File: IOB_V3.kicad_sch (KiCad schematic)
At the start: 6 parts, among them J1 Conn_01x02, J2 Conn_01x03, U1 REF3033

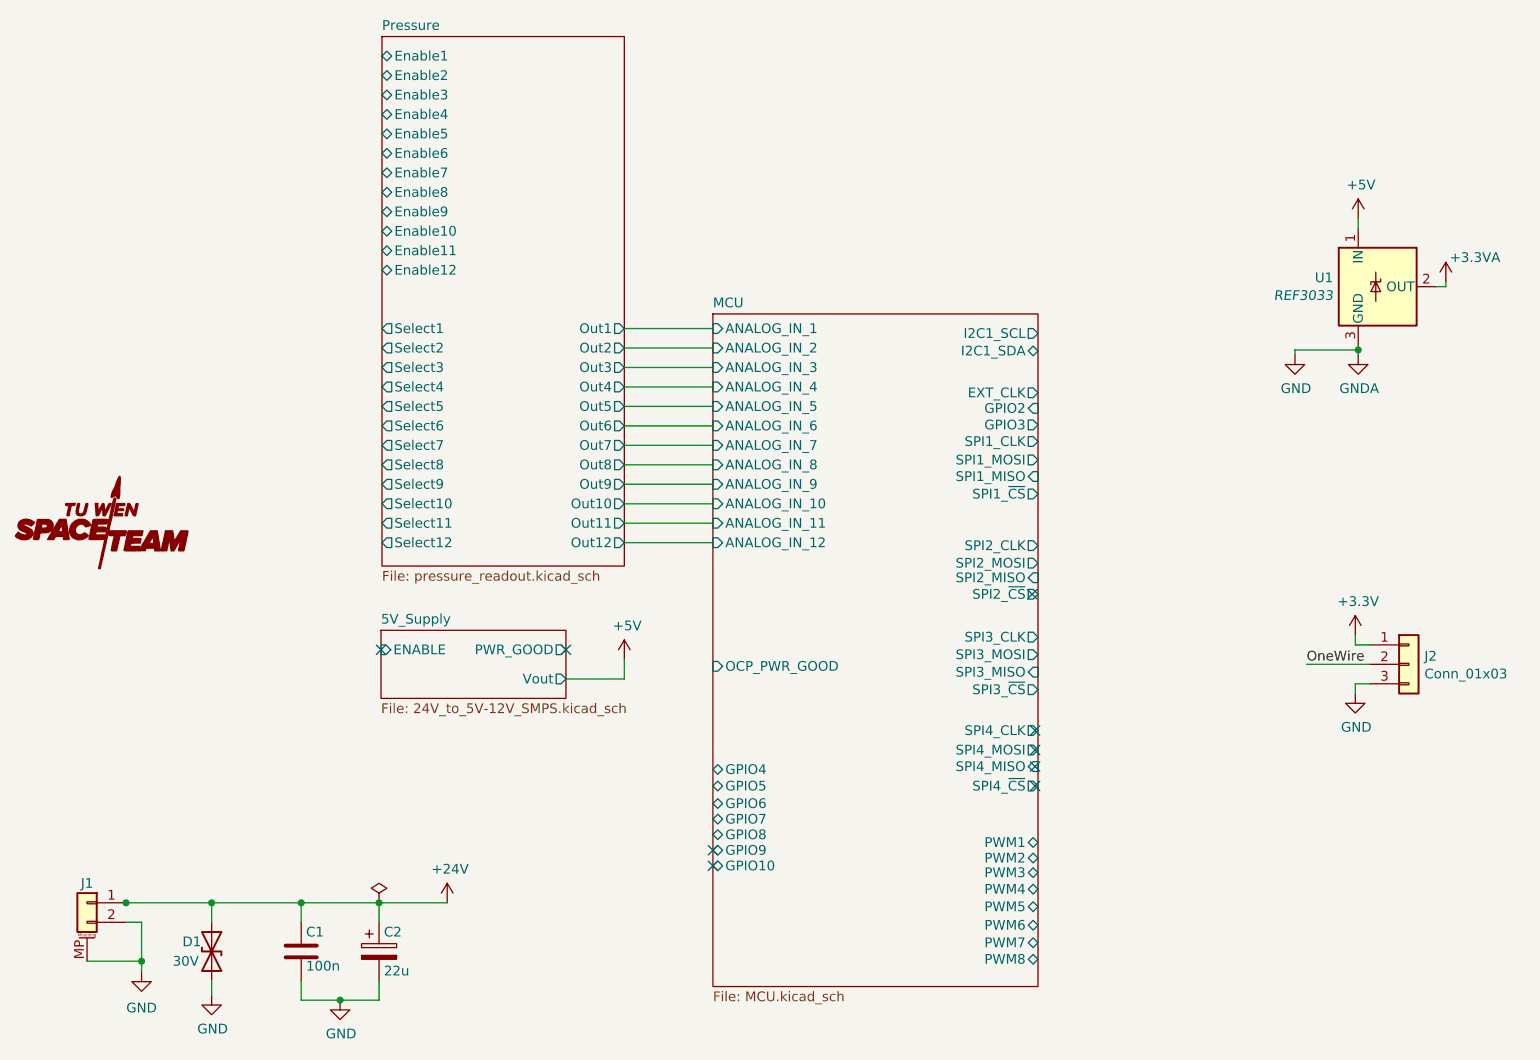
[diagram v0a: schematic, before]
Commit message: WIP
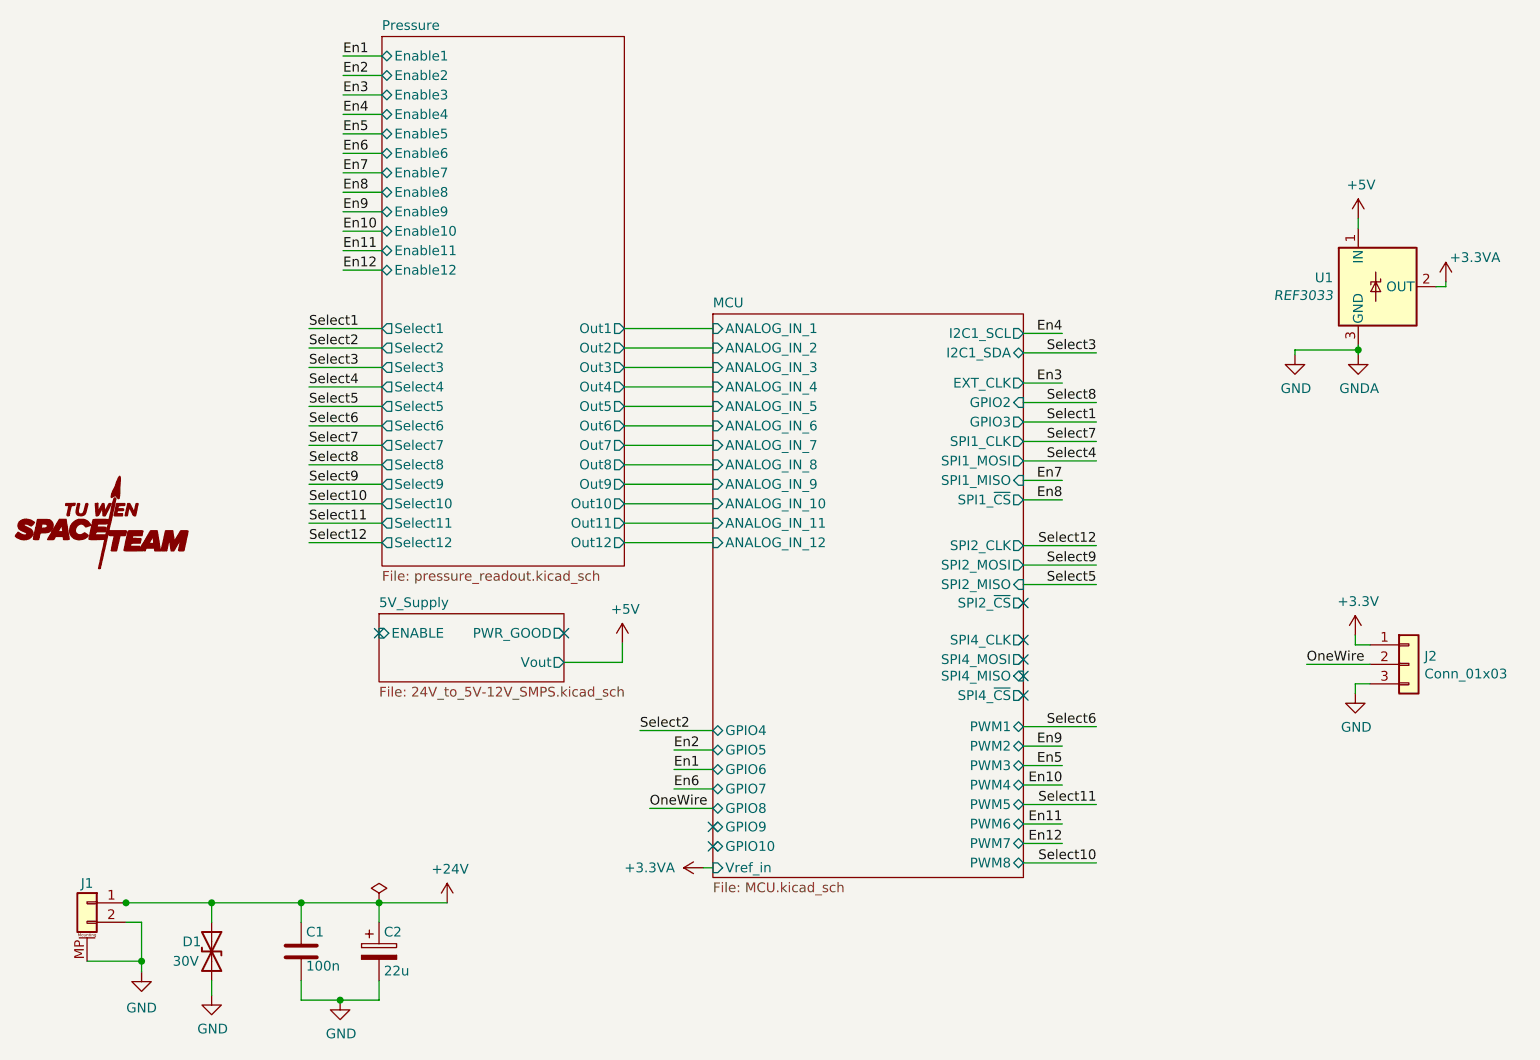
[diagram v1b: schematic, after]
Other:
- sheet MCU ports: added Vref_in; removed OCP_PWR_GOOD, SPI3_CLK, SPI3_MISO, SPI3_MOSI, SPI3_~{CS}
